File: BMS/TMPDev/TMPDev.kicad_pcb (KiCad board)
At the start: 2 copper layers, 52 x 69.8 mm, 7 parts, among them J1 5019510550, J2 5019510550, U1 DS18B20Z+, U13 TMP1075D, U15 TMP1075D

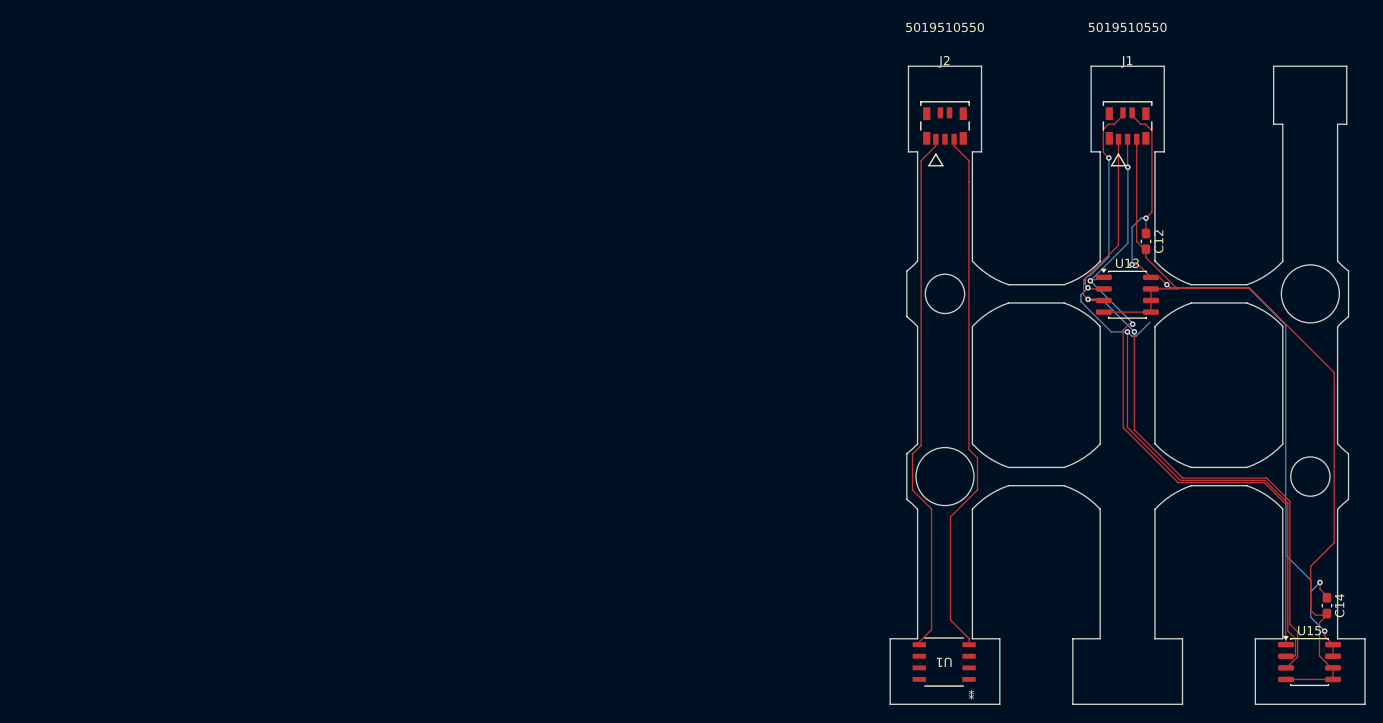
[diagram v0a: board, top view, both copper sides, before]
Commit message: increased size for test module
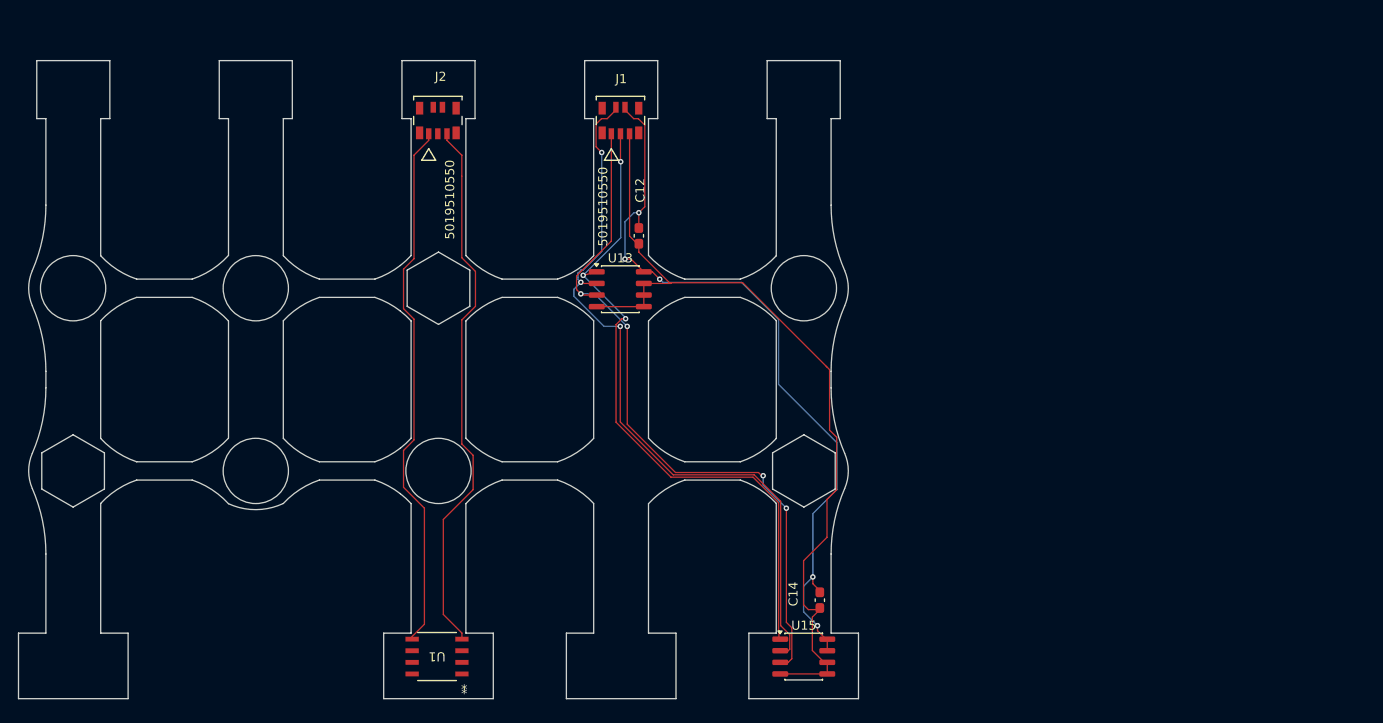
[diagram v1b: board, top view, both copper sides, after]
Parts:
- moved U13 55.5 mm to (91.3, 65.4)
- moved C14 55.5 mm to (113.1, 99.5)
- moved J1 55.5 mm to (91.3, 47.0)
- moved C12 55.5 mm to (93.3, 59.6)
- moved J2 55.5 mm to (71.3, 47.0)
- moved U1 55.5 mm to (71.2, 105.6)
- moved U15 55.4 mm to (111.4, 105.6)
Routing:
- net /SCL: track 84.9 -> 81.4 mm
- net +5V: track 81.8 -> 83.5 mm
- net Net-(U1-DQ): track 58.5 -> 59.9 mm
- net Net-(U1-GND): track 57.8 -> 58.9 mm
- net V-: track 92.4 -> 93.5 mm
- net /ALERT: track 77.8 -> 78.4 mm, vias 2 -> 4
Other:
- board size 52 x 69.8 mm -> 92 x 69.8 mm
